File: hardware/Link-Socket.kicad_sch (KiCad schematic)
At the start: 4 parts, among them J901 NE8FAV, U901 THVD2442

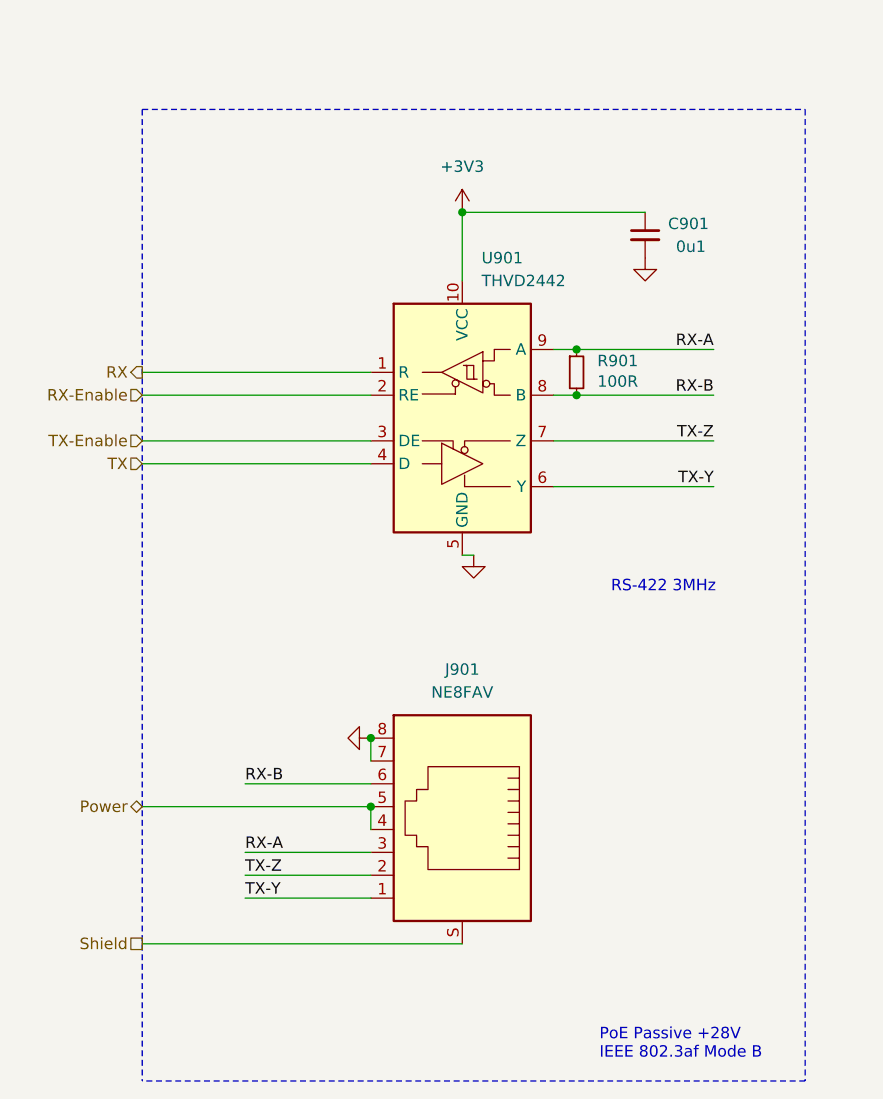
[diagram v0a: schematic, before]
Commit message: Rename
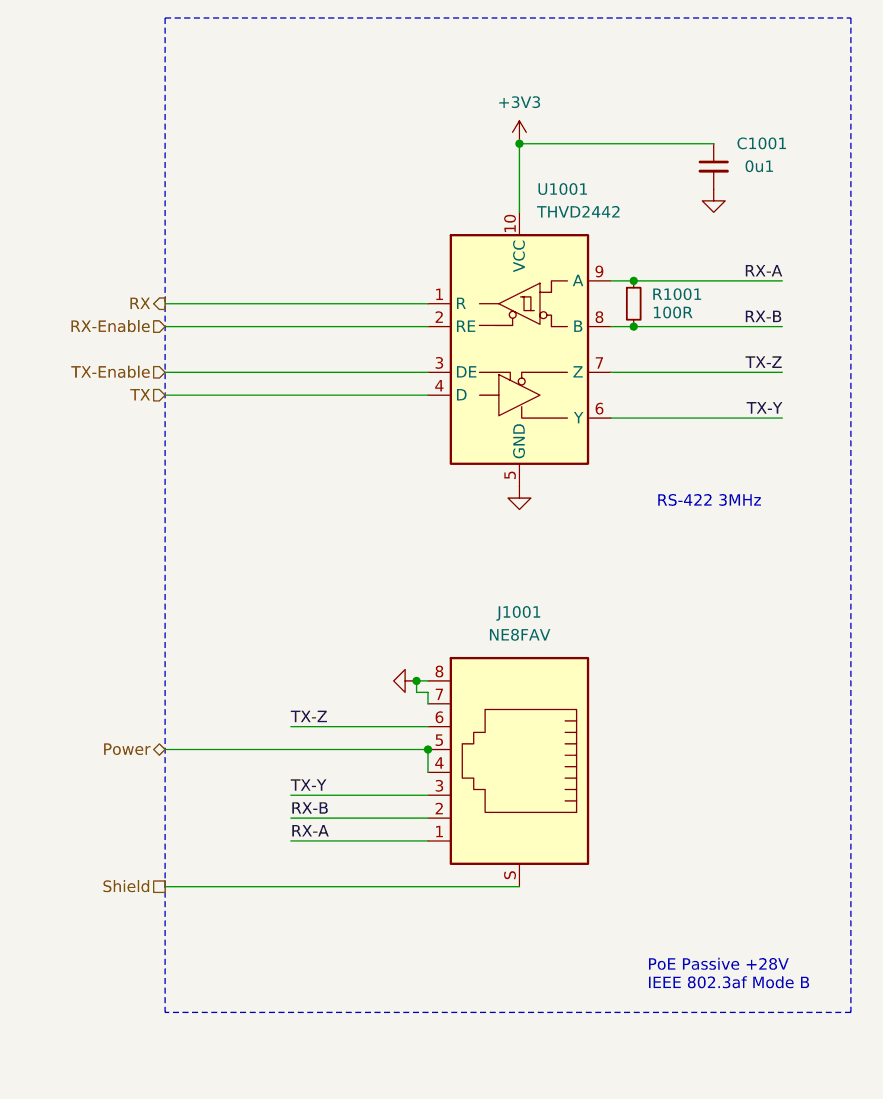
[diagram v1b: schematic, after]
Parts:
- removed C901: 0u1, V2_Capacitor_SMD:C_1608, symbol V2_Capacitor:1608_0u1
- removed J901: NE8FAV, V2_Connector_EtherCon:NE8FAV, symbol V2_Connector_EtherCon:NE8FAV
- removed R901: 100R, V2_Resistor_SMD:R_1608, symbol V2_Resistor:1608_100R
- removed U901: THVD2442, V2_Package_SON:VSON-10-4-1EP_3x3mm_P0.5mm_EP1.65x2.4mm_ThermalVias, symbol V2_Interface_RS485:THVD2442
- added C1001: 0u1, V2_Capacitor_SMD:C_1608, symbol V2_Capacitor:1608_0u1
- added J1001: NE8FAV, V2_Connector_EtherCon:NE8FAV, symbol V2_Connector_EtherCon:NE8FAV
- added R1001: 100R, V2_Resistor_SMD:R_1608, symbol V2_Resistor:1608_100R
- added U1001: THVD2442, V2_Package_SON:VSON-10-4-1EP_3x3mm_P0.5mm_EP1.65x2.4mm_ThermalVias, symbol V2_Interface_RS485:THVD2442
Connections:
- net +3V3: now also C1001.1, U1001.10 (VCC)
- net GND: now also C1001.2, J1001.7, J1001.8, U1001.11 (GND), U1001.5 (GND)
- net Power: now also J1001.4, J1001.5
- net RX: now also U1001.1 (R)
- net RX-A: now also J1001.1, R1001.1, U1001.9 (A)
- net RX-B: now also J1001.2, R1001.2, U1001.8 (B)
- net RX-Enable: now also U1001.2 (RE)
- net Shield: now also J1001.S
- net TX: now also U1001.4 (D)
- net TX-Enable: now also U1001.3 (DE)
- net TX-Y: now also J1001.3, U1001.6 (Y)
- net TX-Z: now also J1001.6, U1001.7 (Z)
